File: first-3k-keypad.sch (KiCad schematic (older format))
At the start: 1 part

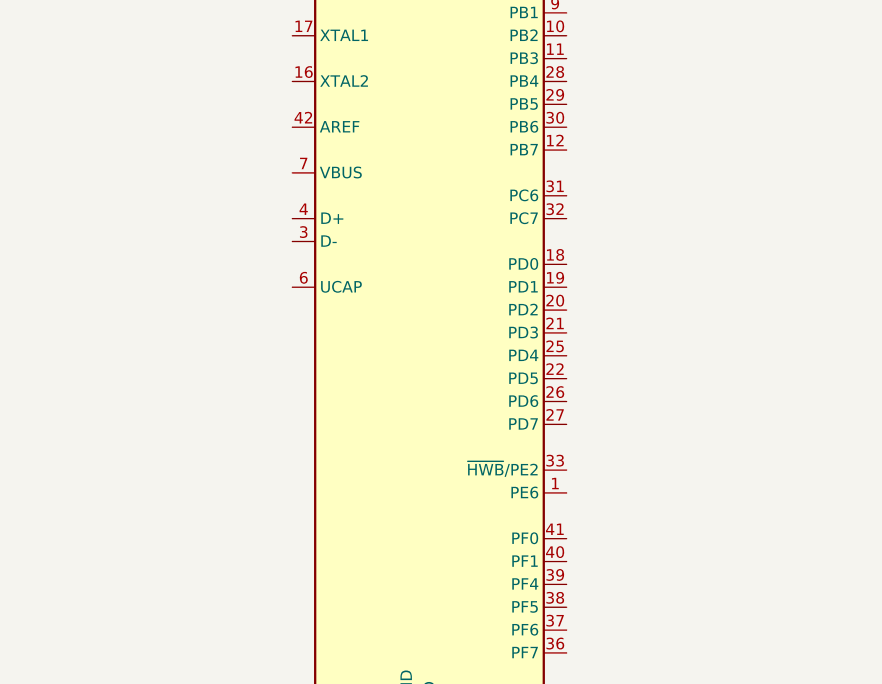
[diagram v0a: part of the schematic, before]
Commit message: 4
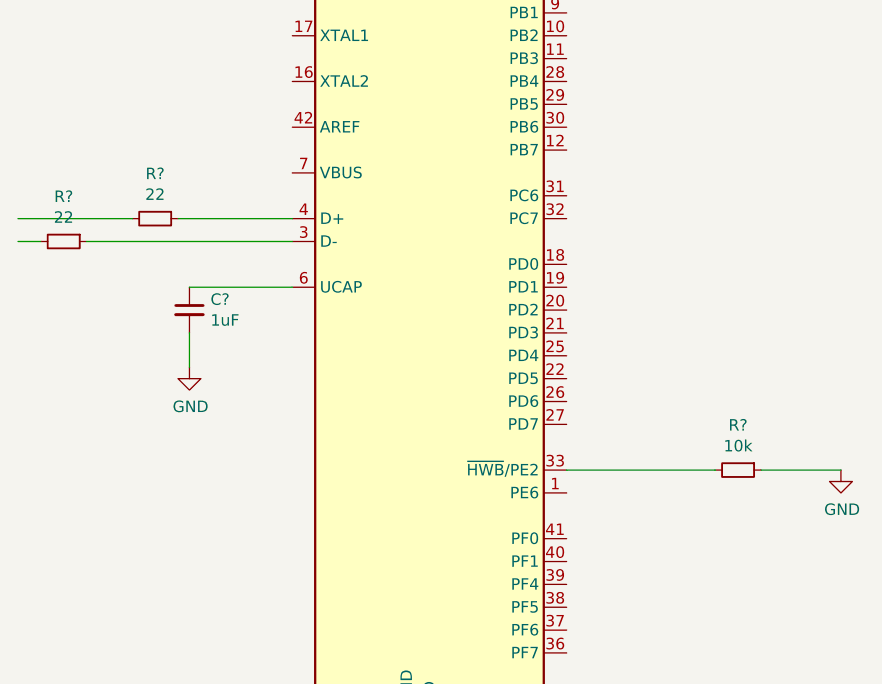
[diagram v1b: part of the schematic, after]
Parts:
- added C?: 1uF, symbol Device:C_Small
- added R?: 10k, symbol Device:R_Small
- added R? (x2): 22, symbol Device:R_Small
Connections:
- wire segments 5 -> 13
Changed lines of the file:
@@
 	5700 5700 5350 5700
 Connection ~ 5700 5700
+$Comp
+L Device:R_Small R?
+U 1 1 634120A0
+P 7150 4500
+F 0 "R?" V 6954 4500 50  0000 C CNN
+F 1 "10k" V 7045 4500 50  0000 C CNN
+F 2 "" H 7150 4500 50  0001 C CNN
+F 3 "~" H 7150 4500 50  0001 C CNN
+	1    7150 4500
+	0    1    1    0
+$EndComp
+$Comp
+L power:GND #PWR?
+U 1 1 63418816
+P 7600 4500
+F 0 "#PWR?" H 7600 4250 50  0001 C CNN
+F 1 "GND" H 7605 4327 50  0000 C CNN
+F 2 "" H 7600 4500 50  0001 C CNN
+F 3 "" H 7600 4500 50  0001 C CNN
+	1    7600 4500
+	1    0    0    -1
+$EndComp
+Wire Wire Line
+	6400 4500 7050 4500
+Wire Wire Line
+	7250 4500 7600 4500
+$Comp
+L Device:R_Small R?
+U 1 1 6341A326
+P 4600 3400
+F 0 "R?" V 4404 3400 50  0000 C CNN
+F 1 "22" V 4495 3400 50  0000 C CNN
+F 2 "" H 4600 3400 50  0001 C CNN
+F 3 "~" H 4600 3400 50  0001 C CNN
+	1    4600 3400
+	0    1    1    0
+$EndComp
+$Comp
+L Device:R_Small R?
+U 1 1 6341B15B
+P 4200 3500
+F 0 "R?" V 4004 3500 50  0000 C CNN
+F 1 "22" V 4095 3500 50  0000 C CNN
+F 2 "" H 4200 3500 50  0001 C CNN
+F 3 "~" H 4200 3500 50  0001 C CNN
+	1    4200 3500
+	0    1    1    0
+$EndComp
+Wire Wire Line
+	5200 3400 4700 3400
+Wire Wire Line
+	5200 3500 4300 3500
+Wire Wire Line
+	4500 3400 4000 3400
+Wire Wire Line
+	4100 3500 4000 3500
+$Comp
+L Device:C_Small C?
+U 1 1 6341E127
+P 4750 3800
+F 0 "C?" H 4842 3846 50  0000 L CNN
+F 1 "1uF" H 4842 3755 50  0000 L CNN
+F 2 "" H 4750 3800 50  0001 C CNN
+F 3 "~" H 4750 3800 50  0001 C CNN
+	1    4750 3800
+	1    0    0    -1
+$EndComp
+Wire Wire Line
+	5200 3700 4750 3700
+$Comp
+L power:GND #PWR?
+U 1 1 634208DE
+P 4750 4050
+F 0 "#PWR?" H 4750 3800 50  0001 C CNN
+F 1 "GND" H 4755 3877 50  0000 C CNN
+F 2 "" H 4750 4050 50  0001 C CNN
+F 3 "" H 4750 4050 50  0001 C CNN
+	1    4750 4050
+	1    0    0    -1
+$EndComp
+Wire Wire Line
+	4750 3900 4750 4050
 $EndSCHEMATC

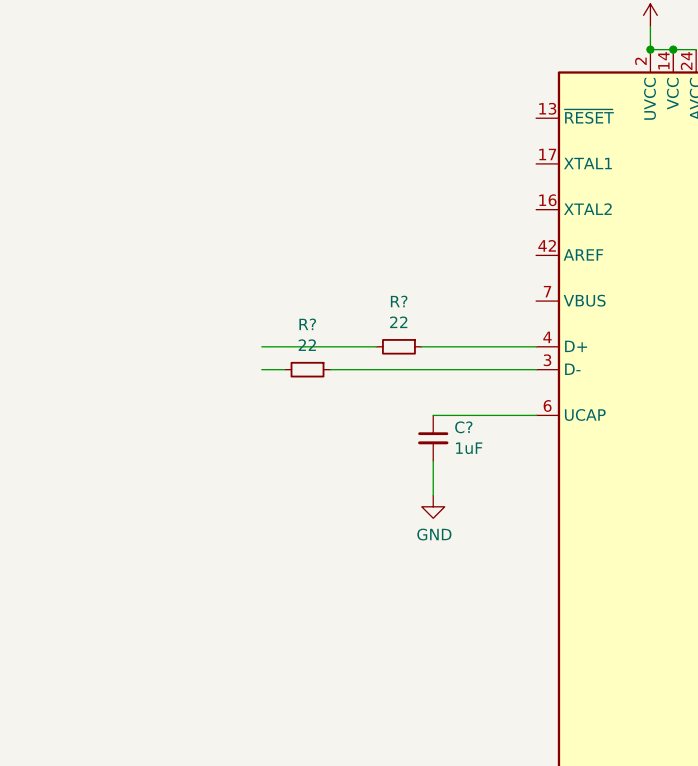
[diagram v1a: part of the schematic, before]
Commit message: 5
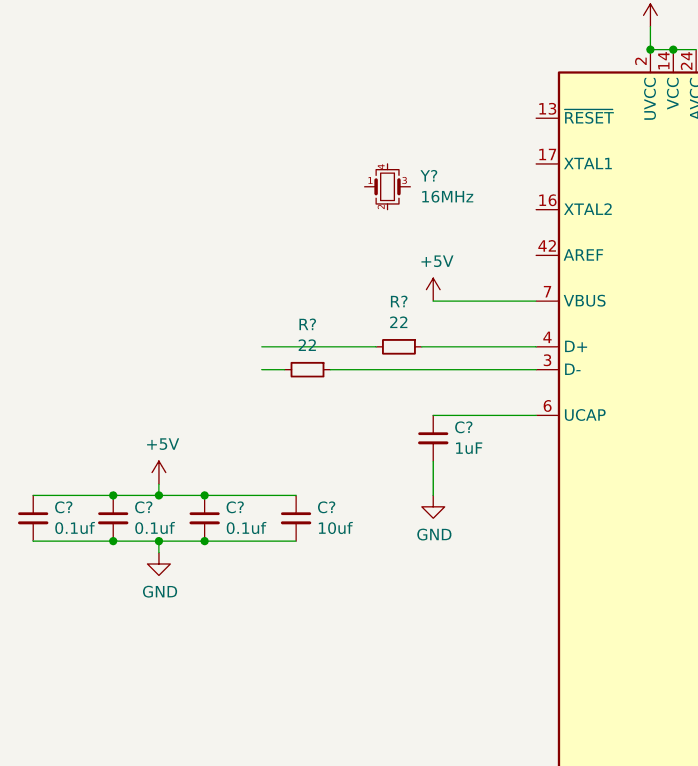
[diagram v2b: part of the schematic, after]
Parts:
- added C? (x3): 0.1uf, symbol Device:C_Small
- added C?: 10uf, symbol Device:C_Small
- added Y?: 16MHz, symbol Device:Crystal_GND24_Small
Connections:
- wire segments 13 -> 24
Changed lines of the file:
@@
 EESchema Schematic File Version 4
+LIBS:first-3k-keypad-cache
 EELAYER 30 0
 EELAYER END
@@
 Wire Wire Line
 	4750 3900 4750 4050
+$Comp
+L Device:C_Small C?
+U 1 1 6351BB14
+P 3000 4150
+F 0 "C?" H 3092 4196 50  0000 L CNN
+F 1 "0.1uf" H 3092 4105 50  0000 L CNN
+F 2 "" H 3000 4150 50  0001 C CNN
+F 3 "~" H 3000 4150 50  0001 C CNN
+	1    3000 4150
+	1    0    0    -1
+$EndComp
+$Comp
+L Device:C_Small C?
+U 1 1 6351E0C3
+P 3350 4150
+F 0 "C?" H 3442 4196 50  0000 L CNN
+F 1 "0.1uf" H 3442 4105 50  0000 L CNN
+F 2 "" H 3350 4150 50  0001 C CNN
+F 3 "~" H 3350 4150 50  0001 C CNN
+	1    3350 4150
+	1    0    0    -1
+$EndComp
+$Comp
+L Device:C_Small C?
+U 1 1 6351EB38
+P 3750 4150
+F 0 "C?" H 3842 4196 50  0000 L CNN
+F 1 "0.1uf" H 3842 4105 50  0000 L CNN
+F 2 "" H 3750 4150 50  0001 C CNN
+F 3 "~" H 3750 4150 50  0001 C CNN
+	1    3750 4150
+	1    0    0    -1
+$EndComp
+$Comp
+L Device:C_Small C?
+U 1 1 6351EE1A
+P 4150 4150
+F 0 "C?" H 4242 4196 50  0000 L CNN
+F 1 "10uf" H 4242 4105 50  0000 L CNN
+F 2 "" H 4150 4150 50  0001 C CNN
+F 3 "~" H 4150 4150 50  0001 C CNN
+	1    4150 4150
+	1    0    0    -1
+$EndComp
+Wire Wire Line
+	3000 4050 3350 4050
+Connection ~ 3350 4050
+Connection ~ 3750 4050
+Wire Wire Line
+	3750 4050 4150 4050
+Wire Wire Line
+	3000 4250 3350 4250
+Connection ~ 3350 4250
+Connection ~ 3750 4250
+Wire Wire Line
+	3750 4250 4150 4250
+Wire Wire Line
+	3350 4050 3550 4050
+Wire Wire Line
+	3350 4250 3550 4250
+Wire Wire Line
+	3550 4050 3550 4000
+Connection ~ 3550 4050
+Wire Wire Line
+	3550 4050 3750 4050
+Wire Wire Line
+	3550 4250 3550 4300
+Connection ~ 3550 4250
+Wire Wire Line
+	3550 4250 3750 4250
+$Comp
+L power:GND #PWR?
+U 1 1 63524E27
+P 3550 4300
+F 0 "#PWR?" H 3550 4050 50  0001 C CNN
+F 1 "GND" H 3555 4127 50  0000 C CNN
+F 2 "" H 3550 4300 50  0001 C CNN
+F 3 "" H 3550 4300 50  0001 C CNN
+	1    3550 4300
+	1    0    0    -1
+$EndComp
+$Comp
+L power:+5V #PWR?
+U 1 1 63525888
+P 3550 4000
+F 0 "#PWR?" H 3550 3850 50  0001 C CNN
+F 1 "+5V" H 3565 4173 50  0000 C CNN
+F 2 "" H 3550 4000 50  0001 C CNN
+F 3 "" H 3550 4000 50  0001 C CNN
+	1    3550 4000
+	1    0    0    -1
+$EndComp
+Wire Wire Line
+	5200 3200 4750 3200
+$Comp
+L power:+5V #PWR?
+U 1 1 63526C97
+P 4750 3200
+F 0 "#PWR?" H 4750 3050 50  0001 C CNN
+F 1 "+5V" H 4765 3373 50  0000 C CNN
+F 2 "" H 4750 3200 50  0001 C CNN
+F 3 "" H 4750 3200 50  0001 C CNN
+	1    4750 3200
+	1    0    0    -1
+$EndComp
+$Comp
+L Device:Crystal_GND24_Small Y?
+U 1 1 6352765E
+P 4550 2700
+F 0 "Y?" H 4694 2746 50  0000 L CNN
+F 1 "16MHz" H 4694 2655 50  0000 L CNN
+F 2 "" H 4550 2700 50  0001 C CNN
+F 3 "~" H 4550 2700 50  0001 C CNN
+	1    4550 2700
+	1    0    0    -1
+$EndComp
 $EndSCHEMATC

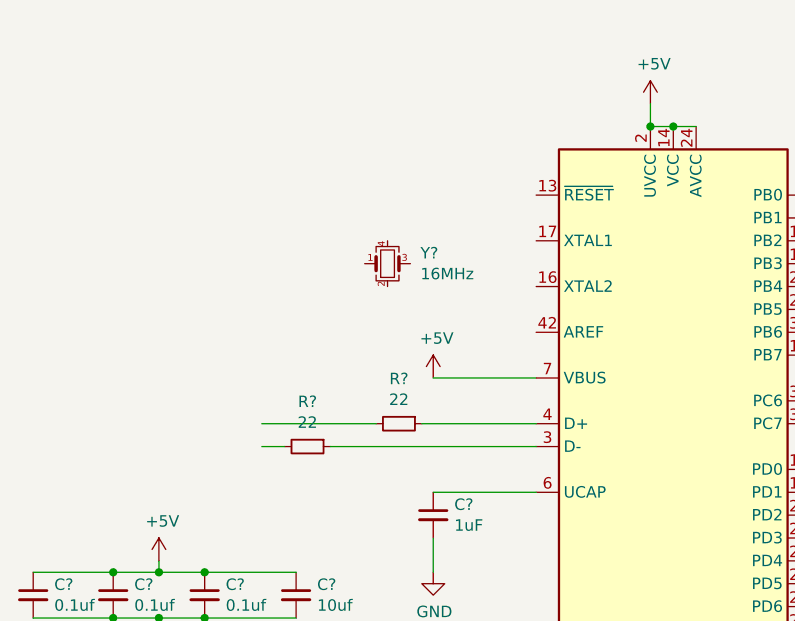
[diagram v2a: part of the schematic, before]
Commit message: 6
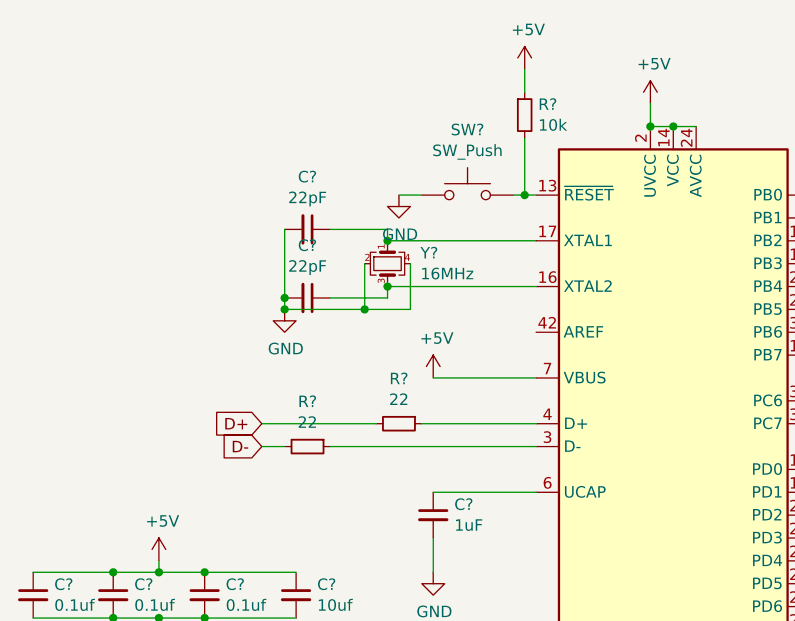
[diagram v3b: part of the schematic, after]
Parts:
- added C? (x2): 22pF, symbol Device:C_Small
- added R?: 10k, symbol Device:R_Small
- added SW?: SW_Push, symbol Switch:SW_Push
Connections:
- net labels added: D+, D-
- wire segments 24 -> 41
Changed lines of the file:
@@
 U 1 1 6352765E
 P 4550 2700
-F 0 "Y?" H 4694 2746 50  0000 L CNN
-F 1 "16MHz" H 4694 2655 50  0000 L CNN
+F 0 "Y?" V 4504 2844 50  0000 L CNN
+F 1 "16MHz" V 4595 2844 50  0000 L CNN
 F 2 "" H 4550 2700 50  0001 C CNN
 F 3 "~" H 4550 2700 50  0001 C CNN
 	1    4550 2700
+	0    1    1    0
+$EndComp
+Wire Wire Line
+	5200 2600 4550 2600
+Wire Wire Line
+	4550 2800 5200 2800
+$Comp
+L power:GND #PWR?
+U 1 1 6352B32F
+P 4100 2900
+F 0 "#PWR?" H 4100 2650 50  0001 C CNN
+F 1 "GND" H 4105 2727 50  0000 C CNN
+F 2 "" H 4100 2900 50  0001 C CNN
+F 3 "" H 4100 2900 50  0001 C CNN
+	1    4100 2900
 	1    0    0    -1
 $EndComp
+$Comp
+L Device:C_Small C?
+U 1 1 6352BF05
+P 4200 2550
+F 0 "C?" V 3971 2550 50  0000 C CNN
+F 1 "22pF" V 4062 2550 50  0000 C CNN
+F 2 "" H 4200 2550 50  0001 C CNN
+F 3 "~" H 4200 2550 50  0001 C CNN
+	1    4200 2550
+	0    1    1    0
+$EndComp
+$Comp
+L Device:C_Small C?
+U 1 1 6352CD4F
+P 4200 2850
+F 0 "C?" V 3971 2850 50  0000 C CNN
+F 1 "22pF" V 4062 2850 50  0000 C CNN
+F 2 "" H 4200 2850 50  0001 C CNN
+F 3 "~" H 4200 2850 50  0001 C CNN
+	1    4200 2850
+	0    1    1    0
+$EndComp
+Wire Wire Line
+	4300 2550 4550 2550
+Wire Wire Line
+	4550 2550 4550 2600
+Connection ~ 4550 2600
+Wire Wire Line
+	4550 2800 4550 2850
+Wire Wire Line
+	4550 2850 4300 2850
+Connection ~ 4550 2800
+Wire Wire Line
+	4100 2550 4100 2850
+Connection ~ 4100 2850
+Wire Wire Line
+	4100 2850 4100 2900
+Wire Wire Line
+	4100 2900 4450 2900
+Wire Wire Line
+	4450 2900 4450 2700
+Connection ~ 4100 2900
+Wire Wire Line
+	4450 2900 4650 2900
+Wire Wire Line
+	4650 2900 4650 2700
+Connection ~ 4450 2900
+$Comp
+L Switch:SW_Push SW?
+U 1 1 6353358D
+P 4900 2400
+F 0 "SW?" H 4900 2685 50  0000 C CNN
+F 1 "SW_Push" H 4900 2594 50  0000 C CNN
+F 2 "" H 4900 2600 50  0001 C CNN
+F 3 "~" H 4900 2600 50  0001 C CNN
+	1    4900 2400
+	1    0    0    -1
+$EndComp
+$Comp
+L power:GND #PWR?
+U 1 1 6353478A
+P 4600 2400
+F 0 "#PWR?" H 4600 2150 50  0001 C CNN
+F 1 "GND" H 4605 2227 50  0000 C CNN
+F 2 "" H 4600 2400 50  0001 C CNN
+F 3 "" H 4600 2400 50  0001 C CNN
+	1    4600 2400
+	1    0    0    -1
+$EndComp
+Wire Wire Line
+	4600 2400 4700 2400
+Wire Wire Line
+	5100 2400 5150 2400
+Wire Wire Line
+	5150 2400 5150 2150
+Connection ~ 5150 2400
+Wire Wire Line
+	5150 2400 5200 2400
+$Comp
+L Device:R_Small R?
+U 1 1 635389FC
+P 5150 2050
+F 0 "R?" H 5209 2096 50  0000 L CNN
+F 1 "10k" H 5209 2005 50  0000 L CNN
+F 2 "" H 5150 2050 50  0001 C CNN
+F 3 "~" H 5150 2050 50  0001 C CNN
+	1    5150 2050
+	1    0    0    -1
+$EndComp
+$Comp
+L power:+5V #PWR?
+U 1 1 6353B908
+P 5150 1850
+F 0 "#PWR?" H 5150 1700 50  0001 C CNN
+F 1 "+5V" H 5165 2023 50  0000 C CNN
+F 2 "" H 5150 1850 50  0001 C CNN
+F 3 "" H 5150 1850 50  0001 C CNN
+	1    5150 1850
+	1    0    0    -1
+$EndComp
+Wire Wire Line
+	5150 1850 5150 1950
+Text GLabel 4000 3400 0    50   Input ~ 0
+D+
+Text GLabel 4000 3500 0    50   Input ~ 0
+D-
 $EndSCHEMATC
